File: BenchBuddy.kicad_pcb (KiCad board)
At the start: 4 copper layers, 166.4 x 64.8 mm, 12 parts, among them K1 RELAY_SPDT 1461069-5, Q1 MMBT3904-7-F, U1 OPTO LTV-816S, U8 MCP4922-E/ST

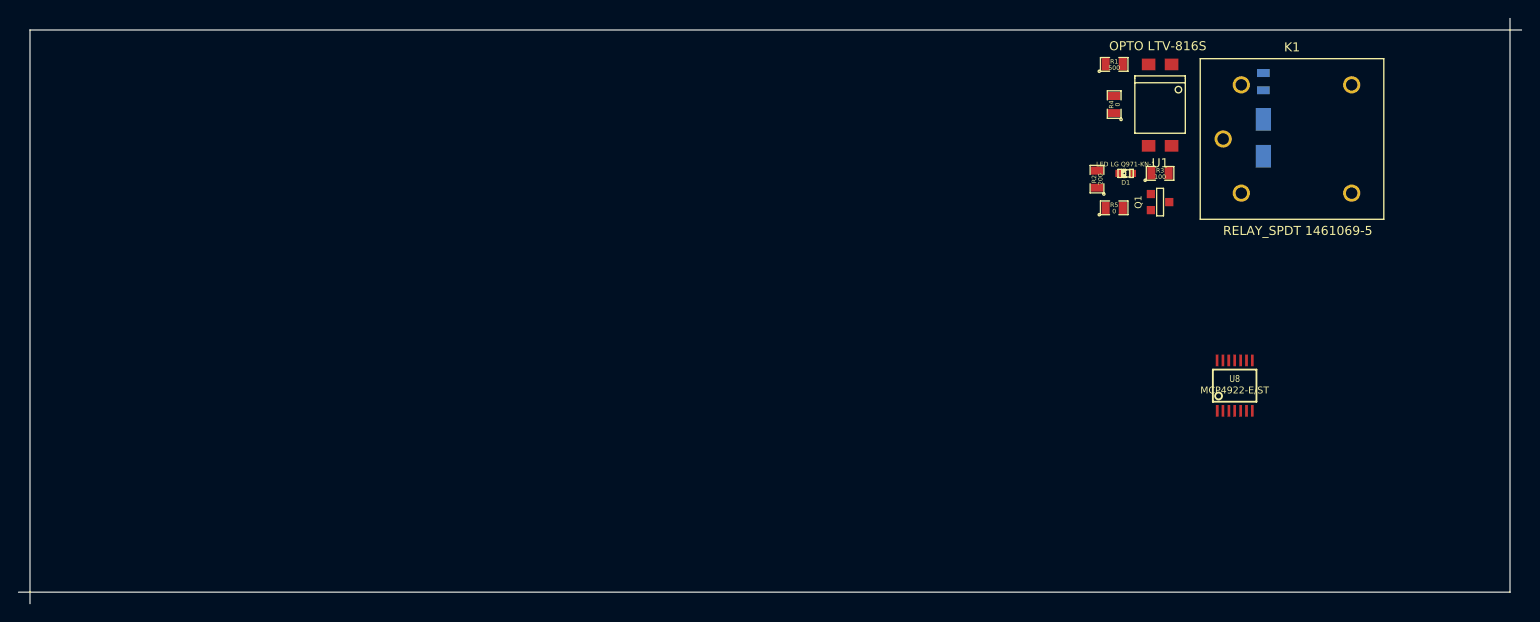
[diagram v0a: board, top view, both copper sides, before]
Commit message: associating-and-placing-the-thermocouple-module
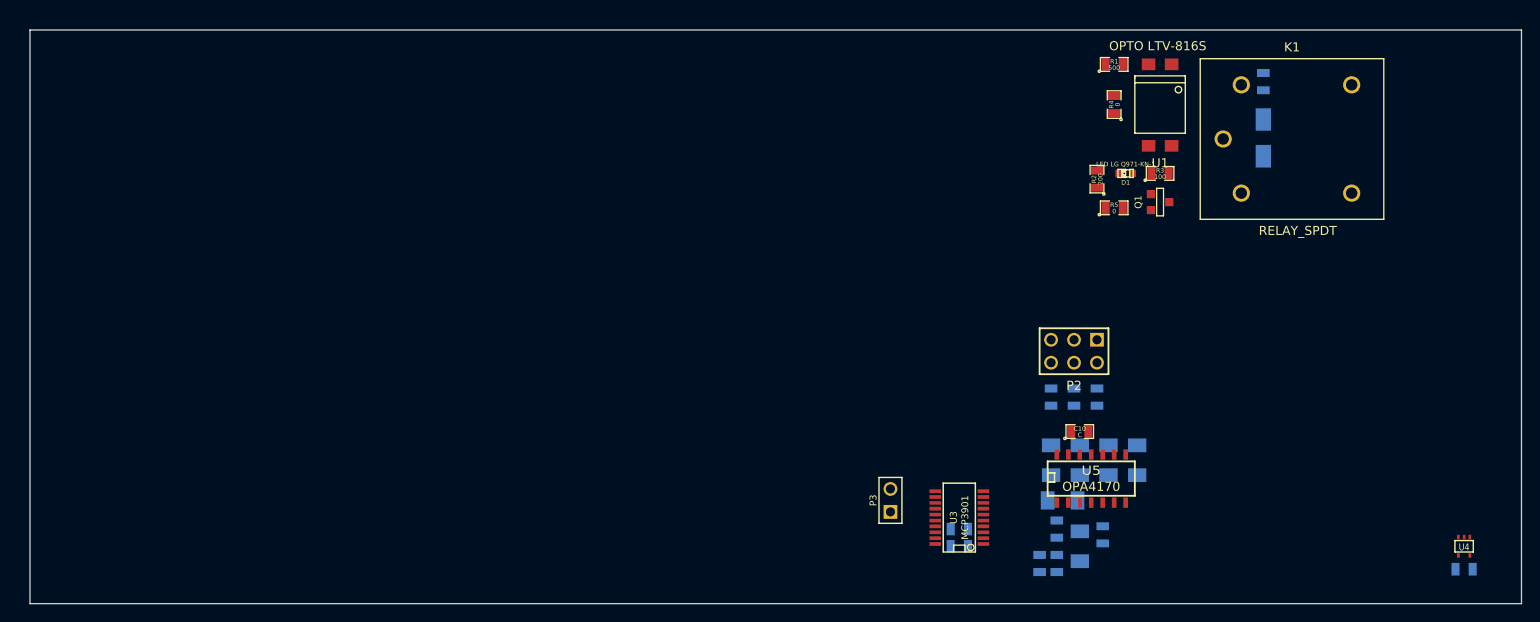
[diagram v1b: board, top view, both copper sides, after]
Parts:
- removed U8: MCP4922-E/ST, TSSOP14
- added C10: C, SM0805, F.Cu at (240.7, 156.2)
- added C11: C, SM0805, B.Cu at (283.2, 171.4)
- added C12: C, SM0805, B.Cu at (243.2, 167.6)
- added C7: C, SM0805, B.Cu at (238.1, 167.0)
- added C8: C, SM0805, B.Cu at (227.3, 168.9)
- added C9: C, SM0805, B.Cu at (227.3, 167.0)
- added P2: CONN_3X2, pin_array_3x2, F.Cu at (240.0, 147.3)
- added P3: CONN_2, PIN_ARRAY_2X1, F.Cu at (219.7, 163.8)
- added R10: R, SM1206, B.Cu at (240.7, 168.9)
- added R11: R, SM1206, B.Cu at (243.8, 159.4)
- added R12: R, SM1206, B.Cu at (237.5, 159.4)
- added R13: R, SM1206, B.Cu at (247.0, 159.4)
- added R14: R, SM0805, B.Cu at (237.5, 152.4)
- added R15: R, SM1206, B.Cu at (240.7, 159.4)
- added R37: R, SM0805, B.Cu at (240.0, 152.4)
- added R38: R, SM0805, B.Cu at (242.6, 152.4)
- added R41: 0, SM0805, B.Cu at (236.2, 170.8)
- added R42: 0, SM0805, B.Cu at (238.1, 170.8)
- added R9: R, SM1206, B.Cu at (238.8, 163.8)
- added U3: MCP3901, SSOP20, F.Cu at (227.3, 165.7)
- added U4: LMT84, SOT353, F.Cu at (283.2, 168.9)
- added U5: OPA4170, SO14E, F.Cu at (241.9, 161.3)
- K1: value RELAY_SPDT 1461069-5 -> RELAY_SPDT
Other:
- board size 166.4 x 64.8 mm -> 165.1 x 63.5 mm
